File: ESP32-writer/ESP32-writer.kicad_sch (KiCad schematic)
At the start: 18 parts, among them J1 USB2.0_C, J2 UART-OUTPUT, J3 USB2.0_C, Q1 2N7002, Q2 2N7002, U1 CH340C, U2 ESP-Prog-ProgramCOM-SEND

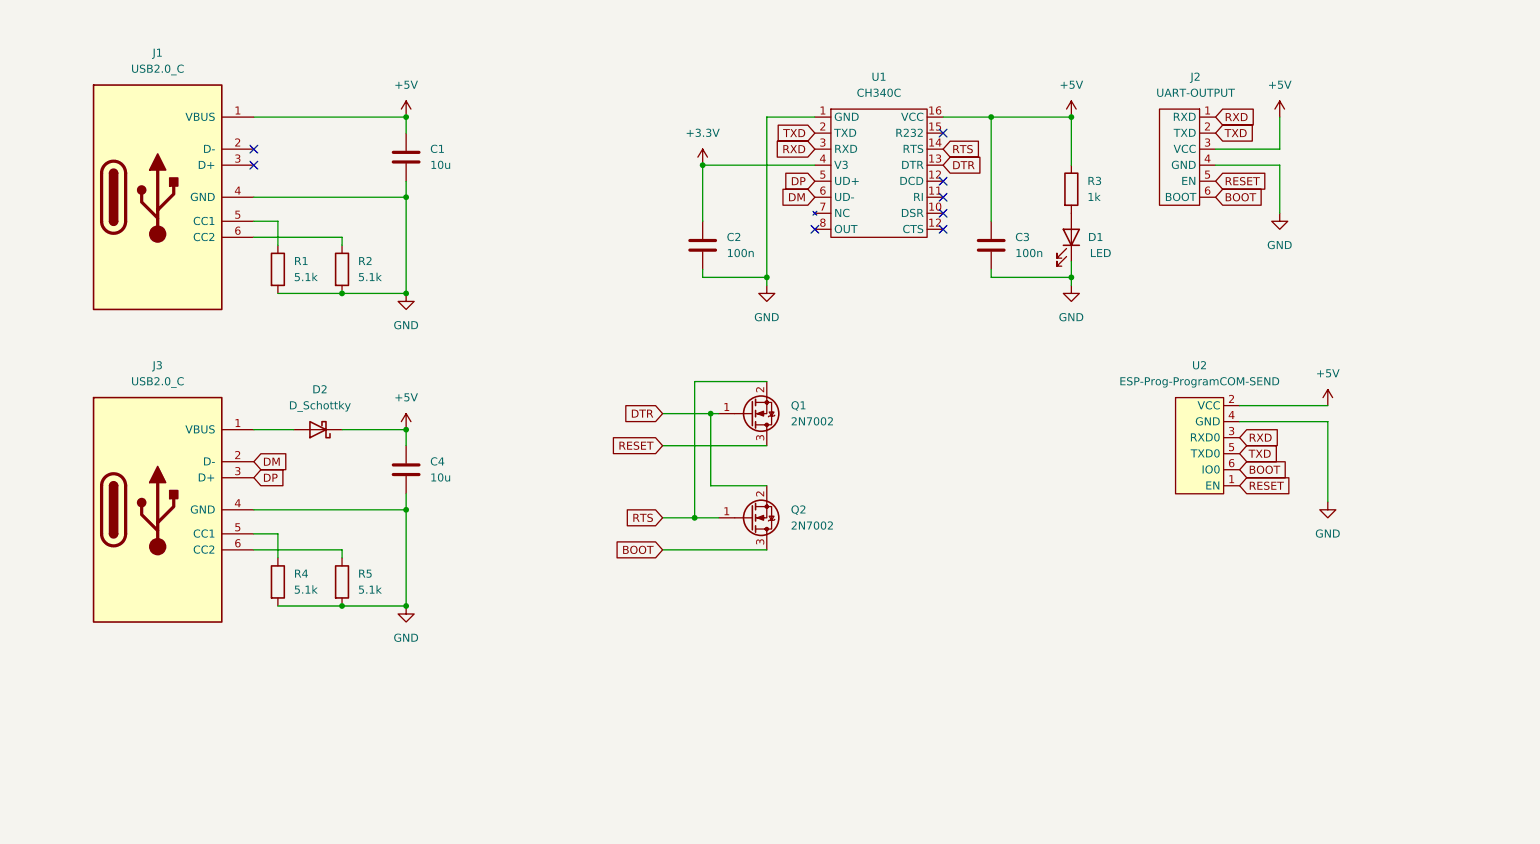
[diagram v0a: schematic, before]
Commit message: update ESP32-Writer
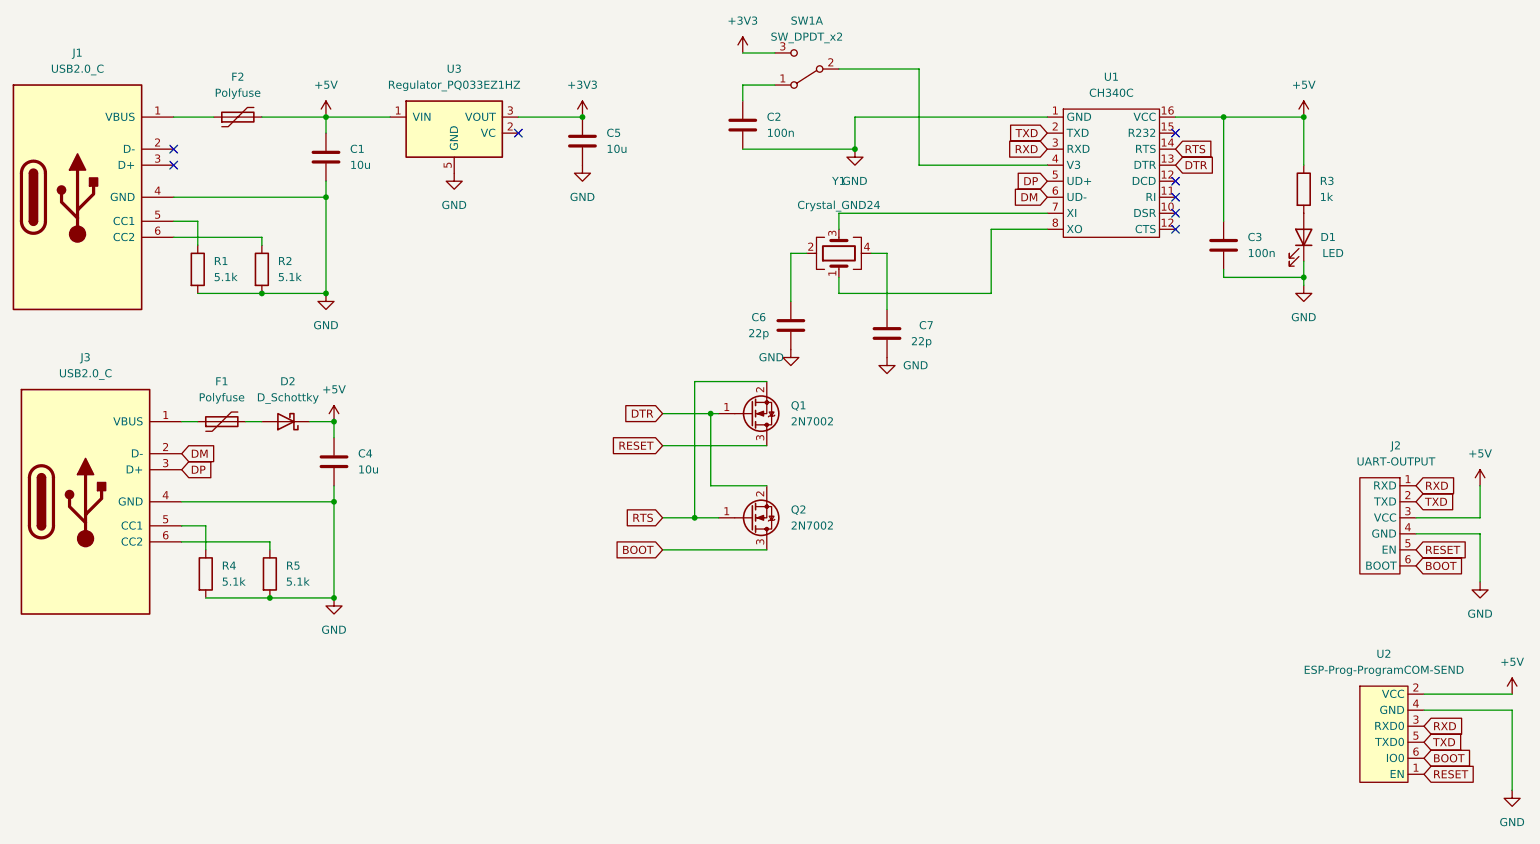
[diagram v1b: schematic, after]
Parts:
- added C5: 10u, $74th:Capacitor_0805_2012, symbol Device:C
- added C6, C7: 22p, $74th:Capacitor_0805_2012, symbol Device:C
- added F1, F2: Polyfuse, symbol Device:Polyfuse
- added SW1: SW_DPDT_x2, symbol Switch:SW_DPDT_x2
- added U3: Regulator_PQ033EZ1HZ, symbol esp32-dev-board:Regulator_PQ033EZ1HZ
- added Y1: Crystal_GND24, symbol Device:Crystal_GND24
- U1: symbol esp32-dev-board:CH340C -> esp32-dev-board:CH340G
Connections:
- net +5V: now also F2.2, U3.1 (VIN); no longer J1.1 (VBUS)
- net GND: now also C5.2, C6.1, C7.1, U3.5 (GND)
- net at D2.2 (A): now also F1.2; no longer J3.1 (VBUS)
- net at U1.7 (XI): now also Y1.3
- net at U1.8 (XO): now also Y1.1
- net +3.3V: no longer names the net of C2.1
- net +3.3V: now also SW1.1 (A); no longer U1.4 (V3)
- new net: C6.2, Y1.2
- new net: C7.2, Y1.4
- new net: F1.1, J3.1 (VBUS)
- new net: SW1.2 (B), U1.4 (V3)
- new net: F2.1, J1.1 (VBUS)
- new net +3V3: C5.1, SW1.3 (C), U3.3 (VOUT)
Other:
- moved on the sheet: C1, C2, C3, C4, D1, D2, J1, J2, J3, R1, R2, R3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

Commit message: up
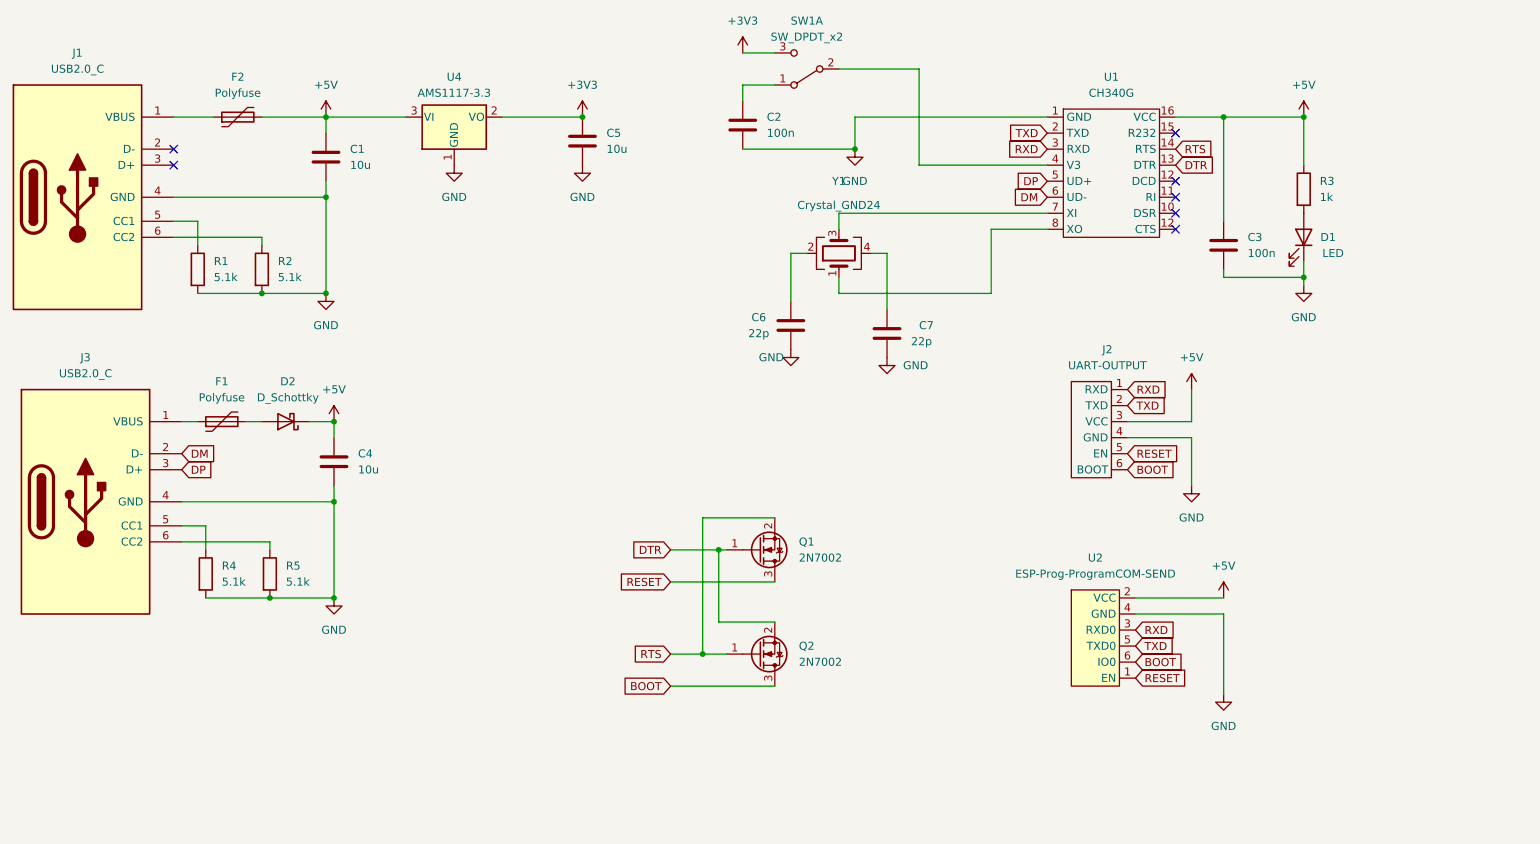
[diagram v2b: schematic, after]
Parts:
- removed U3: Regulator_PQ033EZ1HZ, symbol esp32-dev-board:Regulator_PQ033EZ1HZ
- added U4: AMS1117-3.3, Package_TO_SOT_SMD:SOT-223-3_TabPin2, symbol Regulator_Linear:AMS1117-3.3
- F1, F2: footprint (none) -> $74th:ResettableFuse_KT6-1100SMDI
- U1: value CH340C -> CH340G
- Y1: footprint (none) -> $74th:Crystal_SMD_3215-2Pin_3.2x1.5mm
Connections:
- net +3V3: now also U4.2 (VO)
- net +5V: now also U4.3 (VI)
- net GND: now also U4.1 (GND)
- no-connect marks 8 -> 7
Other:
- moved on the sheet: J2, Q1, Q2, U2
